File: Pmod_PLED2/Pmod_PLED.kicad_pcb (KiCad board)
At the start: 2 copper layers, 22 parts, among them J2 Conn_01x06_Pin, Q1 BSS84, Q2 BSS84, Q4 BSS84, U1 NJW4617, U2 NJW4617, U3 NJW4617

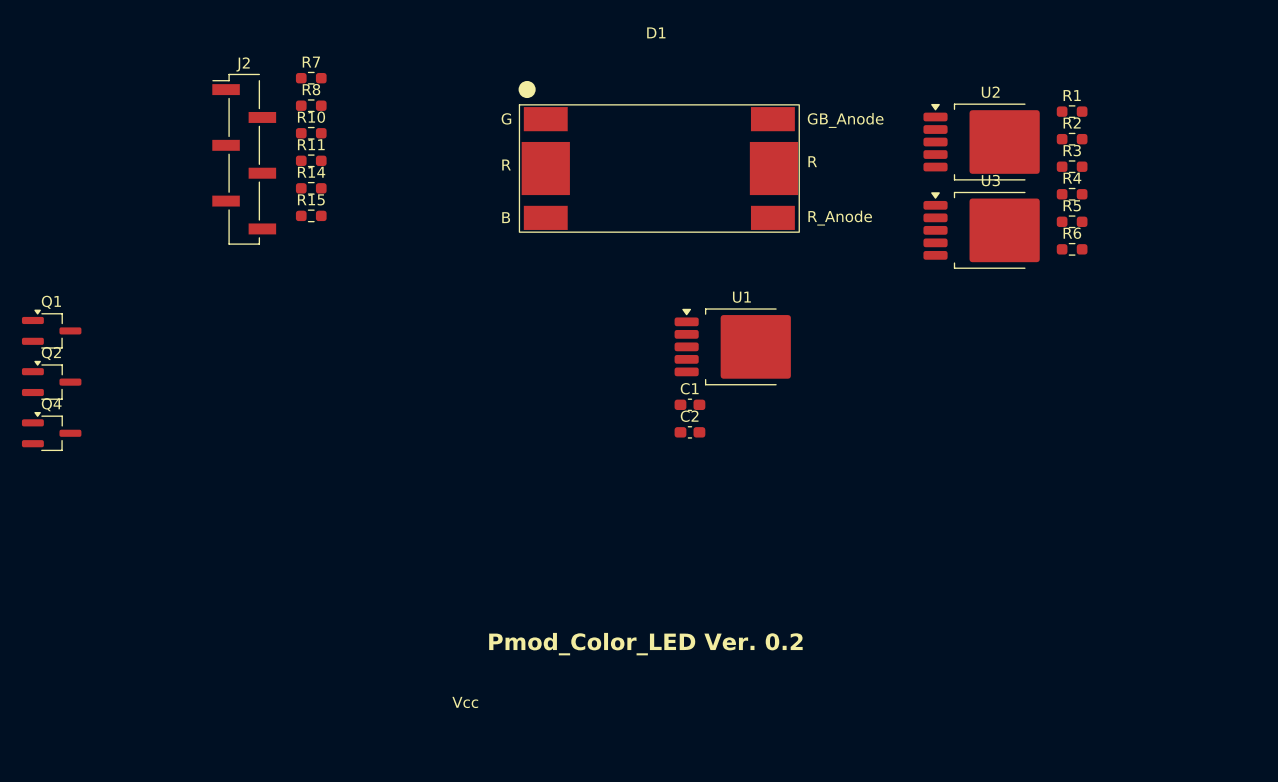
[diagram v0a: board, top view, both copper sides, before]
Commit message: 1110
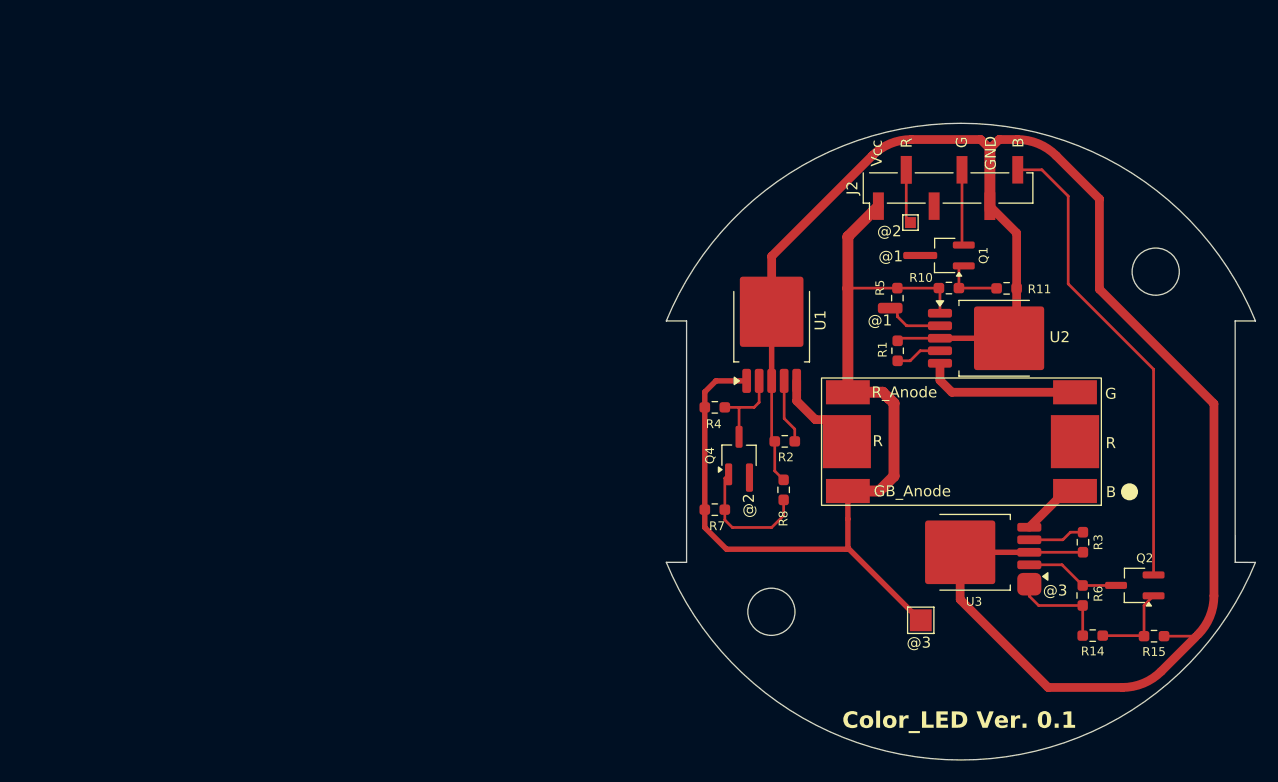
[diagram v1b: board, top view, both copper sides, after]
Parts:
- removed C1, C2: 0.1u, Capacitor_SMD:C_0603_1608Metric_Pad1.08x0.95mm_HandSolder
- added REF**: MountingHole_4.3mm_M4, MountingHole:MountingHole_4.3mm_M4, F.Cu at (124.6, 104.7)
- added REF**: TestPoint_Pad_1.0x1.0mm, TestPoint:TestPoint_Pad_1.0x1.0mm, F.Cu at (137.3, 69.2)
- added REF**: TestPoint_Pad_2.0x2.0mm, TestPoint:TestPoint_Pad_2.0x2.0mm, F.Cu at (138.2, 105.4)
- added REF**: MountingHole_4.3mm_M4, MountingHole:MountingHole_4.3mm_M4, F.Cu at (159.6, 73.7)
- moved Q2 100.4 mm to (157.7, 102.3), turned to 180 degrees
- moved R15 85.8 mm to (159.5, 106.9), turned to 180 degrees
- moved R14 82.1 mm to (153.9, 106.8), turned to 180 degrees
- moved Q1 81.7 mm to (140.4, 72.2), turned to 180 degrees
- moved R11 64.4 mm to (146.0, 75.2), turned to 180 degrees
- moved J2 64.2 mm to (140.7, 66.0), turned to 90 degrees
- moved Q4 62.7 mm to (121.6, 90.4), turned to 90 degrees
- moved R10 59.8 mm to (140.8, 75.2), turned to 180 degrees
- moved R8 55.5 mm to (125.7, 93.5), turned to -90 degrees
- moved R7 53.8 mm to (119.4, 95.4), turned to 180 degrees
- moved R2 38.0 mm to (125.8, 89.1)
- moved R4 37.9 mm to (119.4, 86.0)
- moved D1 37.0 mm to (141.9, 89.2), turned to 180 degrees
- moved R3 34.2 mm to (153.0, 98.3), turned to 90 degrees
- moved R6 31.6 mm to (153.0, 103.2), turned to 90 degrees
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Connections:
- net /Anode_R renamed /Cathode_R
- D1 pad 1: Net-(D1-GK) -> /Cathode_B
- D1 pad 3: /Anode_B -> /Cathode_G
- J2 pad 1: /EN_R -> /5V
- J2 pad 2: /EN_G -> /EN_R
- J2 pad 3: /EN_B -> unconnected-(J2-Pin_3-Pad3)
- J2 pad 4: unconnected-(J2-Pin_4-Pad4) -> /EN_G
- J2 pad 6: /VCC -> /EN_B
- U2 pad 5: Net-(D1-GK) -> /Cathode_G
- U3 pad 5: /Anode_B -> /Cathode_B
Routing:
- net GND: track 0.00 -> 176.3 mm
- net /5V: track 0.00 -> 99.2 mm
- net /EN_B: track 0.00 -> 43.3 mm
- net /Cathode_G: track 0.00 -> 14.3 mm
- net Net-(Q4-G): track 0.00 -> 11.8 mm
- net Net-(Q2-D): track 0.00 -> 8.69 mm
- net Net-(Q4-D): track 0.00 -> 7.96 mm
- net /Cathode_R: track 0.00 -> 7.93 mm
- net Net-(Q2-G): track 0.00 -> 7.82 mm
- net /EN_G: track 0.00 -> 7.01 mm
- net Net-(U1-Rs): track 0.00 -> 5.91 mm
- net /Cathode_B: track 0.00 -> 5.53 mm
- net Net-(Q1-G): track 0.00 -> 5.44 mm
- net Net-(U3-Rs): track 0.00 -> 5.18 mm
- net Net-(Q1-D): track 0.00 -> 5.07 mm
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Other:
- board outline added: 53.7 x 58 mm
- board text added: "@1"
- board text added: "@2"
- board text added: "@3"
- board text added: "B"
- board text added: "Color_LED Ver. 0.1"
- board text added: "G"
- board text added: "GND"
- board text added: "R"
- board text removed: "Pmod_Color_LED Ver. 0.2"
- board text removed: "[EP204K- 150G1R1B1-CA]"
